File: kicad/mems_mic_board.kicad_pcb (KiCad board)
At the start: 2 copper layers, 9 parts, among them J1 Conn_01x08_Male, J2 Conn_01x06_Male, J3 Conn_01x01_Male, J4 Conn_01x10_Male, J5 Conn_01x08_Male, J6 Conn_01x04_Female, U1 tactile_sw, U2 mems_mic, U3 mems_mic

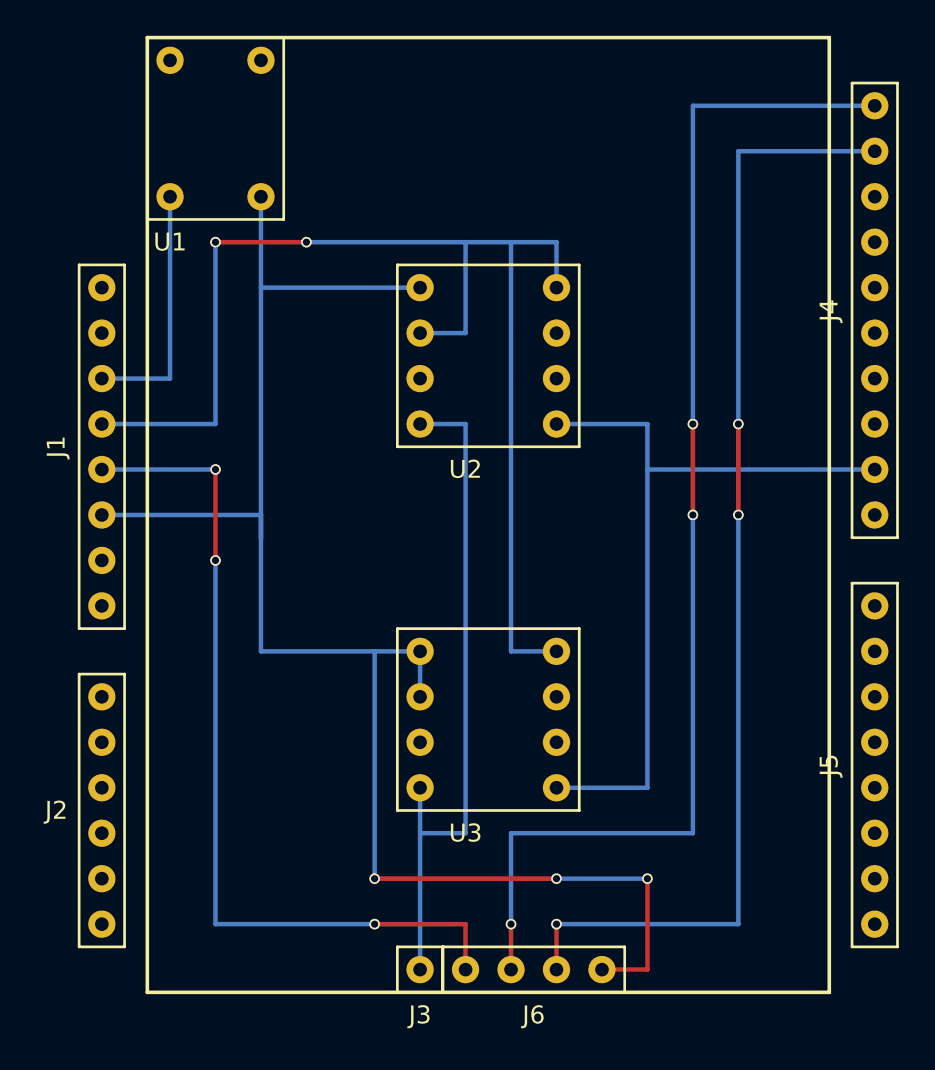
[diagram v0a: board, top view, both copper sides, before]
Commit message: update
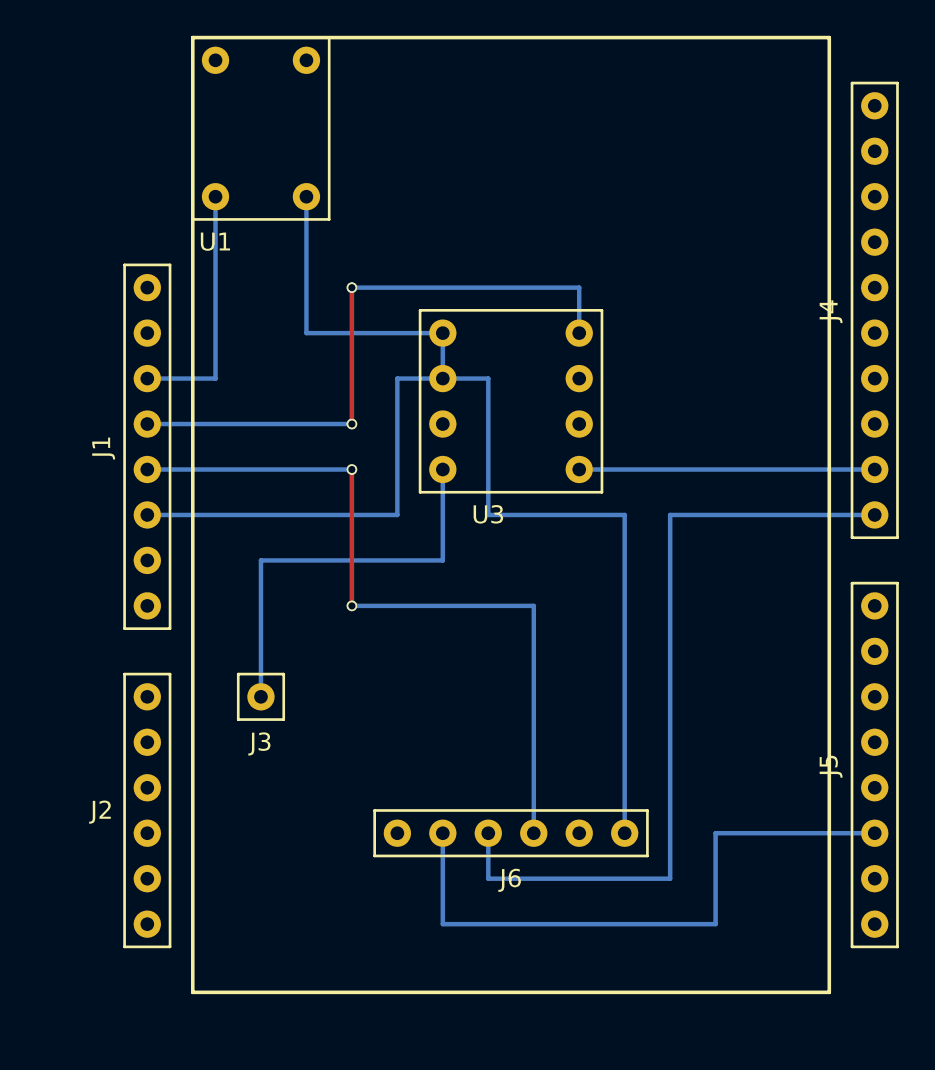
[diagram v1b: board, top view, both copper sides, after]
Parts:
- removed U2: mems_mic, mcu:MEMS_mic
- J6: value Conn_01x04_Female -> Conn_01x06_Female; footprint mcu:pin-socket-4p -> mcu:Pin_Socket_6P
- moved U3 17.8 mm to (134.6, 105.4)
- moved J3 17.6 mm to (120.7, 121.9)
- moved J6 7.73 mm to (134.6, 129.5)
- moved U1 2.54 mm to (120.7, 90.2)
- moved J1 2.54 mm to (114.3, 108.0)
- moved J2 2.54 mm to (114.3, 128.3)
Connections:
- J1 pad 5: /5V -> U5V
- J4 pad 1: /SCL -> Net-(J4-Pad1)
- J4 pad 2: /SDA -> Net-(J4-Pad2)
- J6 pad 1: /5V -> Net-(J6-Pad1)
- J6 pad 2: /SCL -> Net-(J5-Pad6)
- J6 pad 3: /SDA -> Net-(J4-Pad10)
- J6 pad 4: GND -> U5V
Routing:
- net /SCL: track 68.6 -> 0.00 mm, vias 3 -> 0
- net /SDA: track 63.5 -> 0.00 mm, vias 3 -> 0
- net /5V: track 48.3 -> 0.00 mm, vias 3 -> 0
- net Net-(J4-Pad10): track 0.00 -> 44.5 mm
- net U5V: track 0.00 -> 41.9 mm, vias 0 -> 2
- net +3V3: track 71.1 -> 34.3 mm
- net Net-(J5-Pad6): track 0.00 -> 34.3 mm
- net Net-(J4-Pad9): track 43.2 -> 16.5 mm
- net Net-(J3-Pad1): track 38.1 -> 22.9 mm
- net GND: track 91.4 -> 77.5 mm, vias 3 -> 0
